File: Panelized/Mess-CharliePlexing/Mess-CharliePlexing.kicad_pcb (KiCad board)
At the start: 2 copper layers, 98.6 x 99.6 mm, 840 parts, among them J1 Conn_02x19_Odd_Even, J10 Jumper, J11 Jumper, J12 Jumper, J13 Jumper, J14 Jumper, J15 Jumper, J16 Jumper, J17 Jumper, J18 Jumper, J19 Conn_02x19_Odd_Even, J2 Jumper, J20 Jumper, J21 Jumper, J22 Jumper, J23 Jumper, J24 Jumper, J25 Jumper, J26 Jumper, J27 Jumper, J28 Conn_02x19_Odd_Even, J29 Jumper, J3 Jumper, J30 Jumper, J31 Jumper, J32 Jumper, J33 Jumper, J34 Jumper, J35 Jumper, J36 Jumper, J37 Conn_02x19_Odd_Even, J38 Jumper, J39 Jumper, J4 Jumper, J40 Jumper, J41 Jumper, J42 Jumper, J43 Jumper, J44 Jumper, J45 Jumper, J46 Conn_02x19_Odd_Even, J47 Jumper, J48 Jumper, J49 Jumper, J5 Jumper, J50 Jumper, J51 Jumper, J52 Jumper, J53 Jumper, J54 Jumper, J6 Jumper, J7 Jumper, J8 Jumper, J9 Conn_02x19_Odd_Even

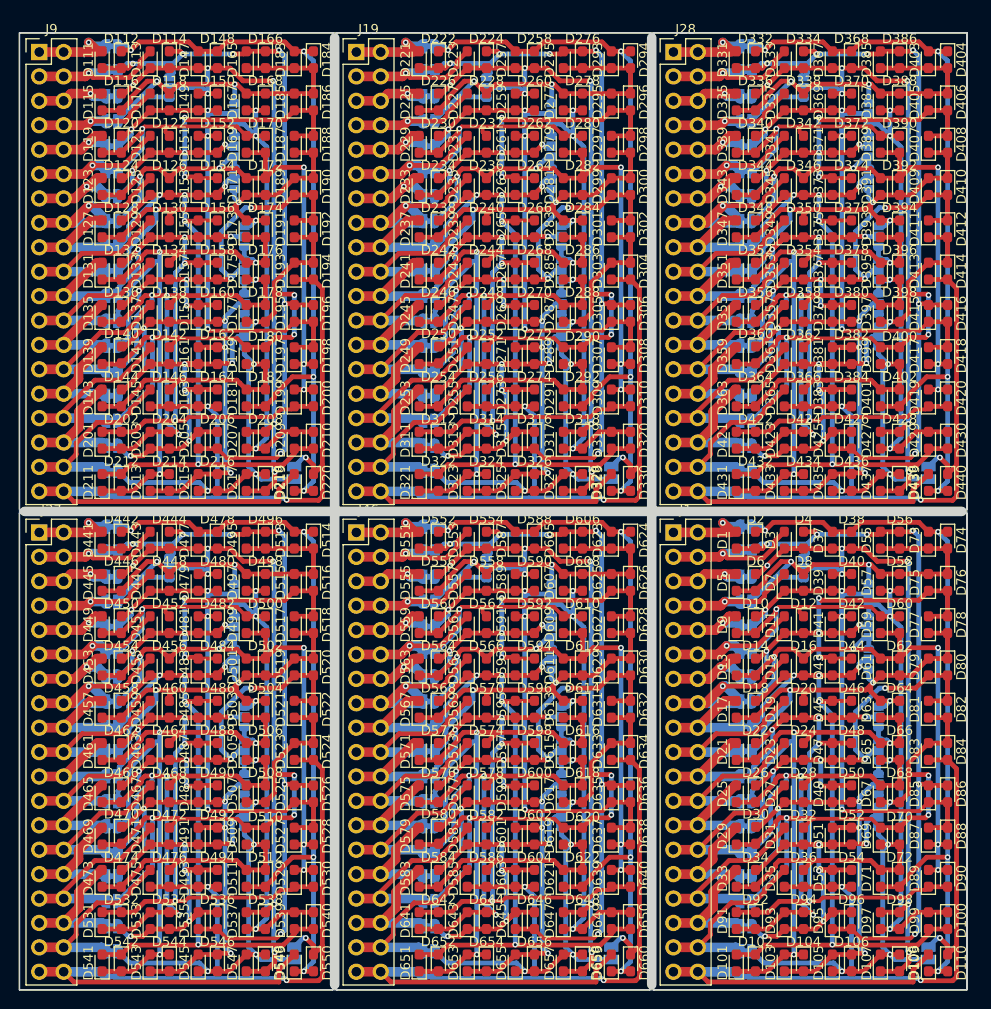
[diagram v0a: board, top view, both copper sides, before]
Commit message: update.
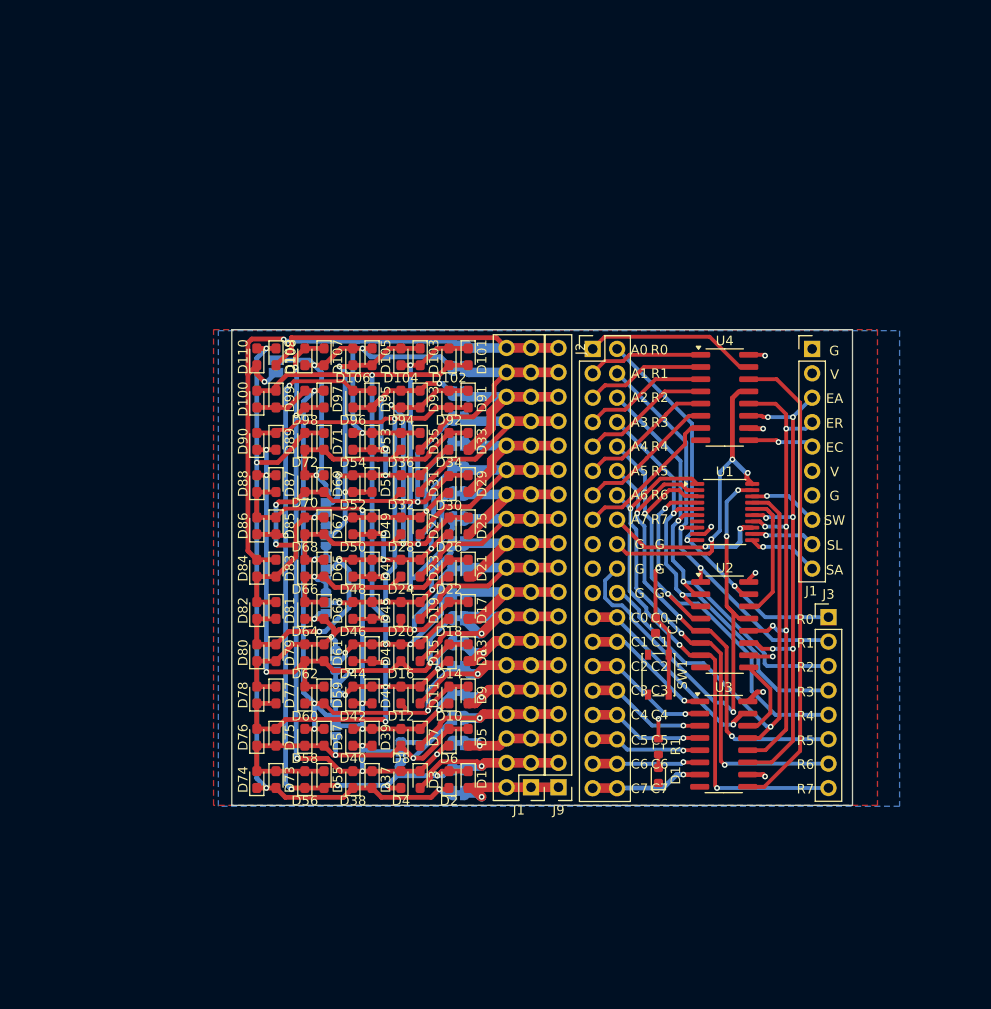
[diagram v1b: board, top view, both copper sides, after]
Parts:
- removed the D1 at (150.4, 101.8)
- removed D111, D112, D113, D114, D115, D116, D117, D118, D119, D120, D121, D122, D123, D124, D125, D126, D127, D128, D129, D130, D131, D132, D133, D134, D135, D136, D137, D138, D139, D140, D141, D142, D143, D144, D145, D146, D147, D148, D149, D150, D151, D152, D153, D154, D155, D156, D157, D158, D159, D160, D161, D162, D163, D164, D165, D166, D167, D168, D169, D170, D171, D172, D173, D174, D175, D176, D177, D178, D179, D180, D181, D182, D183, D184, D185, D186, D187, D188, D189, D190, D191, D192, D193, D194, D195, D196, D197, D198, D199, D200, D201, D202, D203, D204, D205, D206, D207, D208, D209, D210, D211, D212, D213, D214, D215, D216, D217, D218, D219, D220, D221, D222, D223, D224, D225, D226, D227, D228, D229, D230, D231, D232, D233, D234, D235, D236, D237, D238, D239, D240, D241, D242, D243, D244, D245, D246, D247, D248, D249, D250, D251, D252, D253, D254, D255, D256, D257, D258, D259, D260, D261, D262, D263, D264, D265, D266, D267, D268, D269, D270, D271, D272, D273, D274, D275, D276, D277, D278, D279, D280, D281, D282, D283, D284, D285, D286, D287, D288, D289, D290, D291, D292, D293, D294, D295, D296, D297, D298, D299, D300, D301, D302, D303, D304, D305, D306, D307, D308, D309, D310, D311, D312, D313, D314, D315, D316, D317, D318, D319, D320, D321, D322, D323, D324, D325, D326, D327, D328, D329, D330, D331, D332, D333, D334, D335, D336, D337, D338, D339, D340, D341, D342, D343, D344, D345, D346, D347, D348, D349, D350, D351, D352, D353, D354, D355, D356, D357, D358, D359, D360, D361, D362, D363, D364, D365, D366, D367, D368, D369, D370, D371, D372, D373, D374, D375, D376, D377, D378, D379, D380, D381, D382, D383, D384, D385, D386, D387, D388, D389, D390, D391, D392, D393, D394, D395, D396, D397, D398, D399, D400, D401, D402, D403, D404, D405, D406, D407, D408, D409, D410, D411, D412, D413, D414, D415, D416, D417, D418, D419, D420, D421, D422, D423, D424, D425, D426, D427, D428, D429, D430, D431, D432, D433, D434, D435, D436, D437, D438, D439, D440, D441, D442, D443, D444, D445, D446, D447, D448, D449, D450, D451, D452, D453, D454, D455, D456, D457, D458, D459, D460, D461, D462, D463, D464, D465, D466, D467, D468, D469, D470, D471, D472, D473, D474, D475, D476, D477, D478, D479, D480, D481, D482, D483, D484, D485, D486, D487, D488, D489, D490, D491, D492, D493, D494, D495, D496, D497, D498, D499, D500, D501, D502, D503, D504, D505, D506, D507, D508, D509, D510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: LED, LED_SMD:LED_0603_1608Metric_Pad1.05x0.95mm_HandSolder
- removed G***1, G***2, G***3, G***4, G***5: LOGO, IOT-Mess-Footprints:catIcon8x8
- removed the J1 at (143.9, 101.0)
- removed J10, J11, J13, J14, J15, J16, J17, J18, J20, J21, J22, J23, J24, J25, J26, J27, J29, J30, J31, J32, J33, J34, J35, J36, J38, J39, J40, J41, J42, J43, J44, J45, J47, J48, J49, J50, J51, J52, J53, J54: Jumper, IOT-Mess-Footprints:Jumper-3_P1.3mm_Open_RoundedPad1.0x1.5mm
- removed J19, J28, J37, J46: Conn_02x19_Odd_Even, Connector_PinHeader_2.54mm:PinHeader_2x19_P2.54mm_Vertical
- removed the J2 at (164.2, 107.4)
- removed the J3 at (164.2, 110.8)
- removed JP100, JP120, JP40, JP60, JP80: Jumper_2_Open, Jumper:SolderJumper-2_P1.3mm_Open_Pad1.0x1.5mm
- removed JP101, JP102, JP103, JP104, JP105, JP106, JP107, JP108, JP109, JP110, JP111, JP112, JP113, JP114, JP115, JP116, JP117, JP118, JP119, JP21, JP22, JP23, JP24, JP25, JP26, JP27, JP28, JP29, JP30, JP31, JP32, JP33, JP34, JP35, JP36, JP37, JP38, JP39, JP41, JP42, JP43, JP44, JP45, JP46, JP47, JP48, JP49, JP50, JP51, JP52, JP53, JP54, JP55, JP56, JP57, JP58, JP59, JP61, JP62, JP63, JP64, JP65, JP66, JP67, JP68, JP69, JP70, JP71, JP72, JP73, JP74, JP75, JP76, JP77, JP78, JP79, JP81, JP82, JP83, JP84, JP85, JP86, JP87, JP88, JP89, JP90, JP91, JP92, JP93, JP94, JP95, JP96, JP97, JP98, JP99: Jumper, Jumper:SolderJumper-2_P1.3mm_Bridged_RoundedPad1.0x1.5mm
- added C1: .1u, Capacitor_SMD:C_0603_1608Metric, F.Cu at (142.0, 110.7)
- added D1: LED, LED_SMD:LED_0603_1608Metric, F.Cu at (142.3, 126.3)
- added D1: LED, LED_SMD:LED_0603_1608Metric_Pad1.05x0.95mm_HandSolder, F.Cu at (122.5, 126.7)
- added J1: Conn_02x19_Odd_Even, Connector_PinHeader_2.54mm:PinHeader_2x19_P2.54mm_Vertical, F.Cu at (129.0, 127.5)
- added J1: Conn_01x10_Pin, Connector_PinHeader_2.54mm:PinHeader_1x10_P2.54mm_Vertical, F.Cu at (158.3, 81.9)
- added J2: Conn_02x19_Odd_Even, Connector_PinHeader_2.54mm:PinHeader_2x19_P2.54mm_Vertical, F.Cu at (135.5, 81.9)
- added J2: Jumper, IOT-Mess-Footprints:Jumper-3_P1.3mm_Open_RoundedPad1.0x1.5mm, B.Cu at (108.7, 121.1)
- added J3: Conn_01x08_Pin, Connector_PinHeader_2.54mm:PinHeader_1x08_P2.54mm_Vertical, F.Cu at (160.0, 109.8)
- added J3: Jumper, IOT-Mess-Footprints:Jumper-3_P1.3mm_Open_RoundedPad1.0x1.5mm, B.Cu at (108.7, 117.7)
- added R1: R, Resistor_SMD:R_0603_1608Metric, F.Cu at (142.3, 123.3)
- added SW1: SW_Push, Button_Switch_SMD:SW_SPST_PTS810, F.Cu at (142.3, 115.8)
- added U1: ~, Package_SO:TSSOP-20_4.4x6.5mm_P0.65mm, F.Cu at (149.2, 98.9)
- added U2: 74HC595, Package_SO:SOP-16_3.9x9.9mm_P1.27mm, F.Cu at (149.2, 110.6)
- added U3: 74HC595, Package_SO:SOP-16_3.9x9.9mm_P1.27mm, F.Cu at (149.1, 123.0)
- added U4: 74HC595, Package_SO:SOP-16_3.9x9.9mm_P1.27mm, F.Cu at (149.2, 87.0)
- J9: value Conn_02x19_Odd_Even -> Conn_01x19_Pin; footprint Connector_PinHeader_2.54mm:PinHeader_2x19_P2.54mm_Vertical -> Connector_PinHeader_2.54mm:PinHeader_1x19_P2.54mm_Vertical
- moved D110 95.6 mm to (100.5, 82.7), turned to 90 degrees
- moved J9 93.7 mm to (131.9, 127.5), turned to 180 degrees
- moved D109 92.7 mm to (102.5, 82.7), turned to -90 degrees
- moved JP20 91.3 mm to (102.5, 83.7), turned to -90 degrees
- moved D100 90.1 mm to (100.5, 87.1), turned to 90 degrees
- moved D108 88.4 mm to (105.5, 82.7), turned to 90 degrees
- moved D99 86.9 mm to (102.5, 87.1), turned to -90 degrees
- moved D107 85.6 mm to (107.5, 82.7), turned to -90 degrees
- moved D90 85.1 mm to (100.5, 91.5), turned to 90 degrees
- moved D98 82.3 mm to (105.5, 87.1), turned to 90 degrees
- moved D89 81.7 mm to (102.5, 91.5), turned to -90 degrees
- moved D106 81.7 mm to (110.5, 82.7), turned to 90 degrees
- moved D88 80.7 mm to (100.5, 95.9), turned to 90 degrees
- moved D97 79.4 mm to (107.5, 87.1), turned to -90 degrees
- moved D105 79.2 mm to (112.5, 82.7), turned to -90 degrees
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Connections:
- J9 pad 10: /P10 -> /P20
- J9 pad 11: /P12 -> /P22
- J9 pad 12: /P12 -> /P24
- J9 pad 13: /P14 -> /P26
- J9 pad 14: /P14 -> /P28
- J9 pad 15: /P16 -> /P30
- J9 pad 16: /P16 -> /P32
- J9 pad 17: /P18 -> /P34
- J9 pad 18: /P18 -> /P36
- J9 pad 19: /P20 -> /P38
- J9 pad 2: /P2 -> /P4
- J9 pad 3: /P4 -> /P6
- J9 pad 4: /P4 -> /P8
- J9 pad 5: /P6 -> /P10
- J9 pad 6: /P6 -> /P12
- J9 pad 7: /P8 -> /P14
- J9 pad 8: /P8 -> /P16
- J9 pad 9: /P10 -> /P18
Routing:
- net Net-(D109-K): track 482.9 -> 80.5 mm, vias 24 -> 4
- net Net-(D1-K): track 471.9 -> 78.6 mm, vias 36 -> 6
- net Net-(D107-K): track 460.4 -> 76.7 mm, vias 36 -> 6
- net Net-(D100-A): track 455.9 -> 76.0 mm, vias 30 -> 5
- net Net-(D10-A): track 449.2 -> 74.9 mm, vias 24 -> 4
- net Net-(D110-K): track 419.9 -> 70.0 mm, vias 18 -> 3
- net Net-(D19-K): track 414.7 -> 69.1 mm, vias 30 -> 5
- net Net-(D101-K): track 400.4 -> 66.7 mm, vias 18 -> 3
- net Net-(D13-K): track 387.5 -> 64.6 mm, vias 30 -> 5
- net Net-(D105-K): track 363.0 -> 60.5 mm, vias 18 -> 3
- net Net-(D25-K): track 362.5 -> 60.4 mm, vias 24 -> 4
- net Net-(D10-K): track 358.9 -> 59.8 mm, vias 24 -> 4
- net Net-(D29-K): track 352.0 -> 58.7 mm, vias 24 -> 4
- net Net-(D103-K): track 314.0 -> 52.3 mm, vias 24 -> 4
- net Net-(D23-K): track 288.8 -> 48.1 mm, vias 30 -> 5
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- added copper zone on F.Cu, net GND
- added copper zone on B.Cu, net VCC
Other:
- board size 98.6 x 99.6 mm -> 64.6 x 49.5 mm
- board text added: "A0"
- board text added: "A1"
- board text added: "A2"
- board text added: "A3"
- board text added: "A4"
- board text added: "A5"
- board text added: "A6"
- board text added: "A7"
- board text added: "C0"
- board text added: "C1"
- board text added: "C2"
- board text added: "C3"
- board text added: "C4"
- board text added: "C5"
- board text added: "C6"
- board text added: "C7"
- board text added: "EA"
- board text added: "EC"
- board text added: "ER"
- board text added: "G"
- board text added: "IOT_Mess LED595 V2.0 8/19/25"
- board text added: "R0"
- board text added: "R1"
- board text added: "R2"
- board text added: "R3"
- board text added: "R4"
- board text added: "R5"
- board text added: "R6"
- board text added: "R7"
- board text added: "SA"
- board text added: "SL"
- board text added: "SW"
- board text added: "V"
- board text removed: "IOT_Mess Charlieplexing V2.0 8/19/25"
